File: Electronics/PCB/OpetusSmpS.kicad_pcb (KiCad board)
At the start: 4 copper layers, 79 x 71.5 mm, 65 parts, among them J2 KPJX-4S-S, J4 Screw_Terminal_01x10, SW1 SW_SPST, SW3 SW_SPST, U1 AMS1117-3.3, U2 ADIP16-Z-LC-R, U3 SN75C3243PWR, U4 ADIP16-Z-LC-R, U5 ADIP10-Z-LC-R

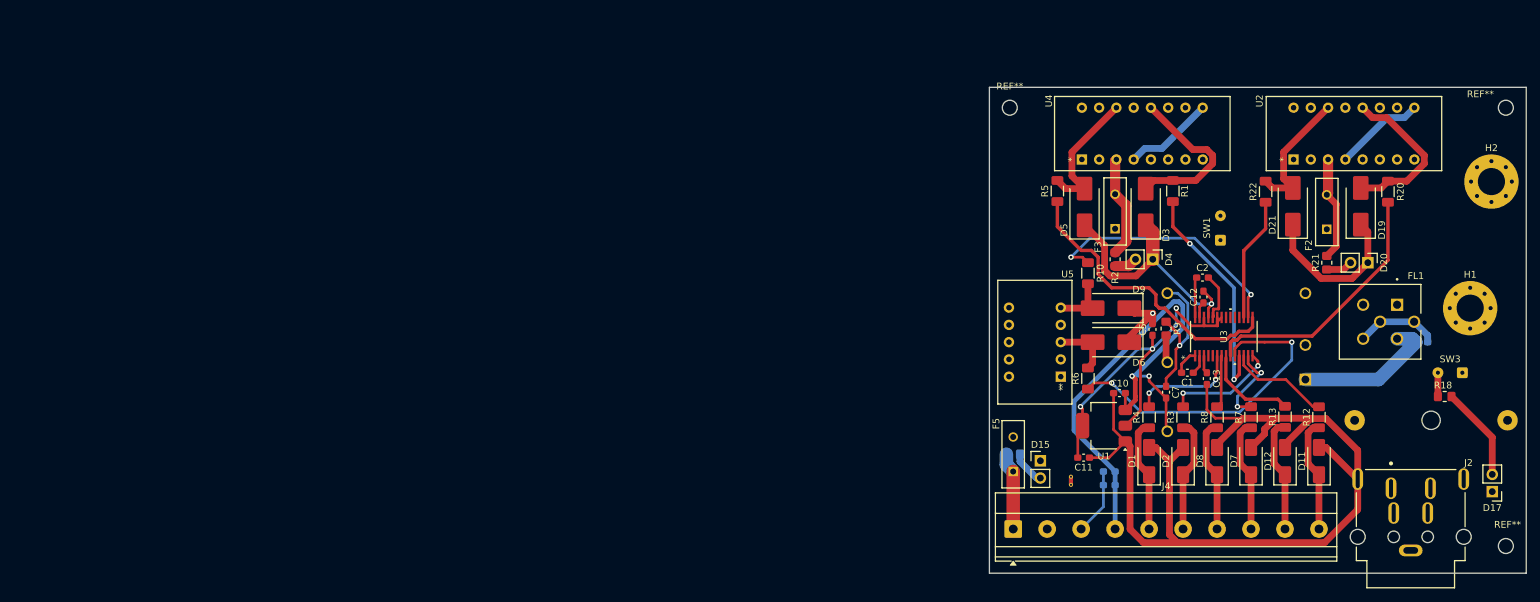
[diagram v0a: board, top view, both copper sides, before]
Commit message: Refactor code structure for improved readability and maintainability
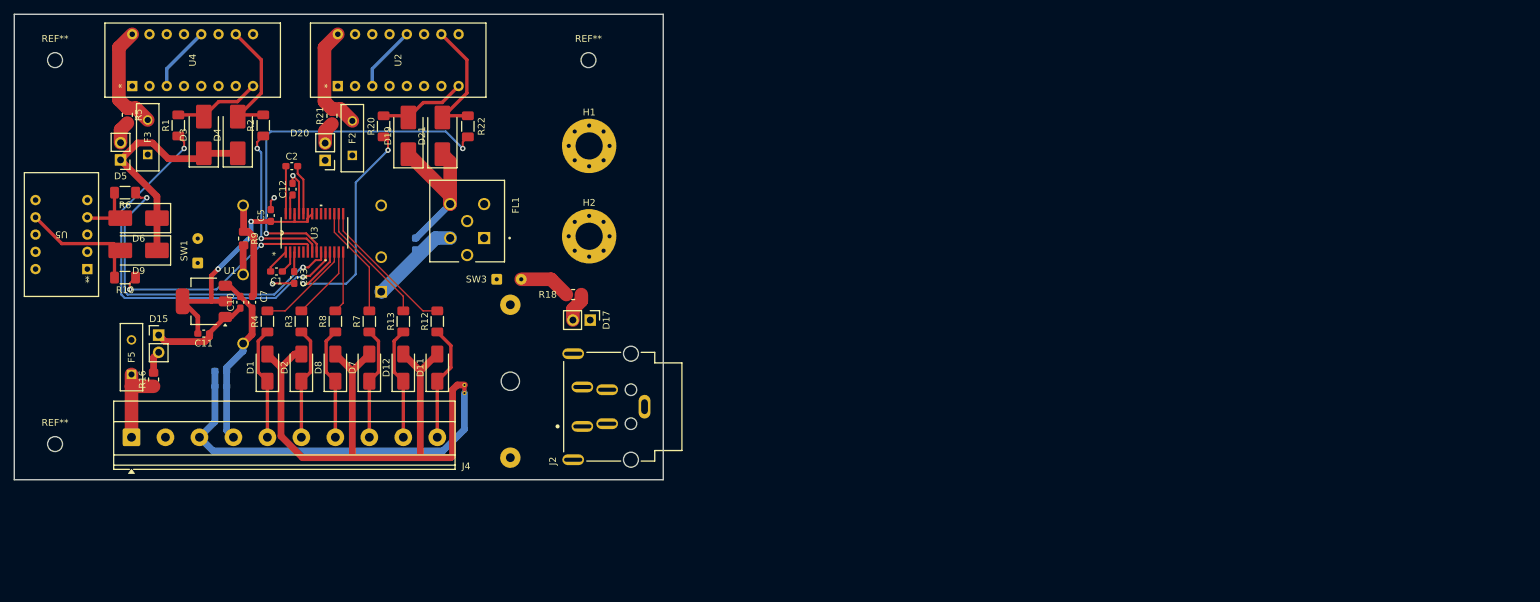
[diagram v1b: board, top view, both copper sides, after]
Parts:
- removed the REF** at (126.0, 63.5)
- removed the REF** at (199.0, 128.0)
- removed the REF** at (199.0, 63.5)
- added REF**: MountingHole_2.2mm_M2, MountingHole:MountingHole_2.2mm_M2, F.Cu at (-14.5, 56.5)
- added REF**: MountingHole_2.2mm_M2, MountingHole:MountingHole_2.2mm_M2, F.Cu at (64.0, 56.5)
- added REF**: MountingHole_2.2mm_M2, MountingHole:MountingHole_2.2mm_M2, F.Cu at (-14.5, 113.0)
- D4: value LED -> 15V; footprint Connector_PinHeader_2.54mm:PinHeader_1x02_P2.54mm_Vertical -> Diode_SMD:D_SMB_Handsoldering
- D5: value 15V -> LED; footprint Diode_SMD:D_SMB_Handsoldering -> Connector_PinHeader_2.54mm:PinHeader_1x02_P2.54mm_Vertical
- R16: moved to F.Cu
- R2: value 10k -> 220; footprint Resistor_SMD:R_0805_2012Metric_Pad1.20x1.40mm_HandSolder -> Resistor_SMD:R_1206_3216Metric_Pad1.30x1.75mm_HandSolder
- R5: value 220 -> 10k; footprint Resistor_SMD:R_1206_3216Metric_Pad1.30x1.75mm_HandSolder -> Resistor_SMD:R_0805_2012Metric_Pad1.20x1.40mm_HandSolder
- moved D20 154.2 mm to (25.2, 71.2), turned to 180 degrees
- moved SW1 150.5 mm to (6.50, 86.3)
- moved C4 148.8 mm to (38.5, 83.5), turned to 90 degrees
- moved R20 148.1 mm to (33.9, 66.2)
- moved R21 148.0 mm to (26.2, 64.7)
- moved R1 146.7 mm to (3.64, 66.1)
- moved R6 144.3 mm to (-4.20, 76.0), turned to 180 degrees
- moved D6 144.2 mm to (-2.20, 79.8)
- moved U5 144.1 mm to (-9.75, 87.2)
- moved F2 143.8 mm to (29.2, 70.5)
- moved D9 143.3 mm to (-2.20, 84.5)
- moved F3 142.8 mm to (-0.86, 70.4)
- moved SW3 142.8 mm to (50.5, 88.8), turned to 0 degrees
- moved D5 142.0 mm to (-4.86, 71.2), turned to 180 degrees
- moved R10 141.7 mm to (-4.20, 88.5), turned to 180 degrees
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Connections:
- D4 pad 2: Net-(D4-A) -> Net-(D4-A2)
- D5 pad 2: Net-(D5-A2) -> Net-(D5-A)
- R1 pad 1: /TX3_OUT -> /TX2_OUT
- R10 pad 1: /RX2_OUT -> /RX_OUT
- R12 pad 2: /TX3_IN -> /RX3_IN
- R13 pad 2: /RX3_IN -> /RX2_IN
- R2 pad 1: Net-(F3-Pad2) -> /RX2_OUT
- R2 pad 2: Net-(D4-A) -> Net-(D4-A2)
- R20 pad 1: /TX_OUT -> /TX3_OUT
- R22 pad 1: /RX_OUT -> /RX3_OUT
- R3 pad 2: /TX_IN -> /TX2_IN
- R4 pad 2: /RX_IN -> /TX3_IN
- R5 pad 1: /RX3_OUT -> Net-(F3-Pad2)
- R5 pad 2: Net-(D5-A2) -> Net-(D5-A)
- R6 pad 1: /TX2_OUT -> /TX_OUT
- R7 pad 2: /TX2_IN -> /RX_IN
- R8 pad 2: /RX2_IN -> /TX_IN
- U2 pad 10: unconnected-(U2-Pad10) -> Net-(D21-A2)
- U2 pad 11: unconnected-(U2-Pad11) -> GND
- U2 pad 12: Net-(D19-A2) -> Net-(U2-Pad12)
- U2 pad 14: Net-(D21-A2) -> unconnected-(U2-Pad14)
- U2 pad 16: unconnected-(U2-Pad16) -> Net-(F2-Pad2)
- U2 pad 3: Net-(F2-Pad2) -> Net-(U2-Pad12)
- U2 pad 4: Net-(U2-Pad4) -> unconnected-(U2-Pad4)
- U2 pad 8: GND -> Net-(D19-A2)
- U2 pad 9: Net-(U2-Pad4) -> unconnected-(U2-Pad9)
- U3 pad 15: /RX3_OUT -> /RX3_IN
- U3 pad 16: /RX2_OUT -> /RX2_IN
- U3 pad 17: /RX_OUT -> /RX_IN
- U3 pad 6: /RX_IN -> /RX_OUT
- U3 pad 7: /RX2_IN -> /RX2_OUT
- U3 pad 8: /RX3_IN -> /RX3_OUT
- U4 pad 10: unconnected-(U4-Pad10) -> Net-(D4-A2)
- U4 pad 11: unconnected-(U4-Pad11) -> GND
- U4 pad 12: Net-(D3-A2) -> Net-(U4-Pad12)
- U4 pad 14: Net-(D5-A2) -> unconnected-(U4-Pad14)
- U4 pad 16: unconnected-(U4-Pad16) -> Net-(F3-Pad2)
- U4 pad 3: Net-(F3-Pad2) -> Net-(U4-Pad12)
- U4 pad 4: Net-(U4-Pad4) -> unconnected-(U4-Pad4)
- U4 pad 8: GND -> Net-(D3-A2)
- U4 pad 9: Net-(U4-Pad4) -> unconnected-(U4-Pad9)
- U5 pad 1: GND -> unconnected-(U5-Pad1)
- U5 pad 3: Net-(D6-A2) -> GND
- U5 pad 4: unconnected-(U5-Pad4) -> Net-(D6-A2)
- U5 pad 5: Net-(D9-A2) -> GND
- U5 pad 7: unconnected-(U5-Pad7) -> Net-(D9-A2)
- U5 pad 9: GND -> unconnected-(U5-Pad9)
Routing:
- net GND: track 646.1 -> 300.3 mm, vias 2 -> 3
- net SGND: track 50.1 -> 108.5 mm, vias 1 -> 0
- net /5V1: track 77.3 -> 26.3 mm, vias 2 -> 0
- net Net-(D5-A2): track 19.9 -> 0.00 mm
- net Net-(D4-A2): track 0.00 -> 19.0 mm
- net Net-(F1-Pad1): track 0.00 -> 18.3 mm
- net /3V3: track 55.8 -> 38.4 mm, vias 3 -> 2
- net /RX_OUT: track 18.3 -> 32.2 mm, vias 0 -> 2
- net /TX2_OUT: track 47.8 -> 61.3 mm
- net Net-(U4-Pad4): track 13.3 -> 0.00 mm
- net Net-(U2-Pad4): track 13.3 -> 0.00 mm
- net /RX2_OUT: track 37.5 -> 24.7 mm
- net /RX3_OUT: track 43.7 -> 55.8 mm, vias 0 -> 2
- net /24OUT: track 72.3 -> 60.6 mm
- net Net-(D3-A2): track 24.6 -> 13.0 mm
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- added copper zone on In1.Cu, net GND
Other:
- board size 79 x 71.5 mm -> 95.5 x 68.5 mm
- board text added: "Teaching smps V2 AYK 8.3.2026"
- board text removed: "Teaching SMPS AYK 14.01.2026"
